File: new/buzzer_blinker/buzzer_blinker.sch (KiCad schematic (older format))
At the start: 9 parts

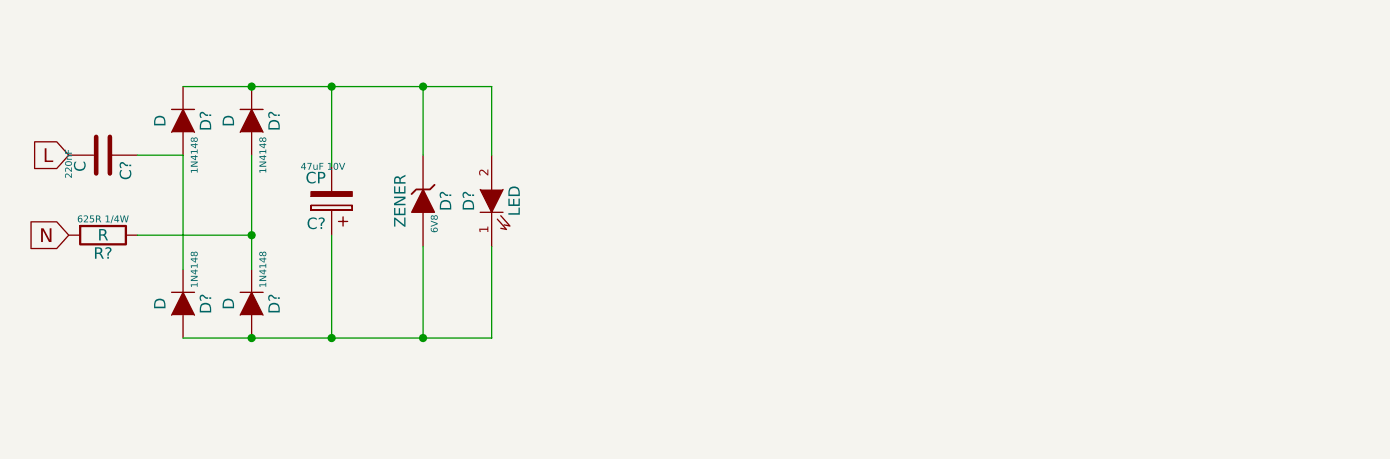
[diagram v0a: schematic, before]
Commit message: .
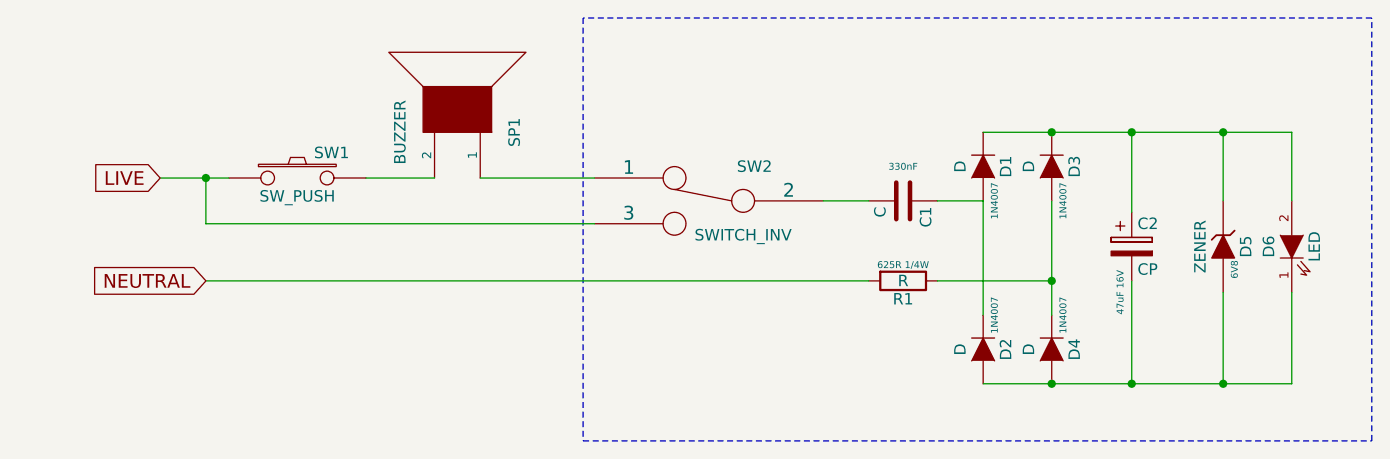
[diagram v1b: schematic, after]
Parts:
- added SP1: BUZZER, symbol SPEAKER
- added SW1: SW_PUSH, symbol SW_PUSH
- added SW2: SWITCH_INV, symbol SWITCH_INV
- C1: renamed from C?; footprint 220nF -> 330nF
- C2: renamed from C?; footprint 47uF 10V -> 47uF 16V
- D1, D2, D3, D4: renamed from D?; footprint 1N4148 -> 1N4007
- gave numbers to parts that had none: 3
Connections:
- net at D1.1 (K), D3.1 (K), D5.1 (K)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: now also C2.1; no longer C2.2
- net at D2.2 (A), D4.2 (A), D5.2 (A)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: now also C2.2; no longer C2.1
- net L: no longer names the net of C1.2
- net L: now also SW2.2
- net N renamed NEUTRAL
- new net: SP1.1, SW2.1
- new net: SP1.2, SW1.2
- new net LIVE: SW1.1, SW2.3
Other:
- moved on the sheet: C1, C2, D1, D2, D3, D4, D5, D6, R1
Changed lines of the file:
@@
 LIBS:contrib
 LIBS:valves
+LIBS:switch_dpdt
+LIBS:buzzer_blinker-cache
 EELAYER 25 0
 EELAYER END
@@
 $EndDescr
 $Comp
-L C C?
+L C C1
 U 1 1 5657A47F
-P 1350 1600
-F 0 "C?" H 1375 1700 50  0000 L CNN
-F 1 "C" H 1375 1500 50  0000 L CNN
-F 2 "220nF" H 1388 1450 30  0000 C CNN
-F 3 "" H 1350 1600 60  0000 C CNN
-	1    1350 1600
-	0    1    1    0
-$EndComp
-$Comp
-L R R?
+P 4850 1800
+F 0 "C1" H 4875 1900 50  0000 L CNN
+F 1 "C" H 4875 1700 50  0000 L CNN
+F 2 "330nF" V 4700 1800 30  0000 C CNN
+F 3 "" H 4850 1800 60  0000 C CNN
+	1    4850 1800
+	0    1    1    0
+$EndComp
+$Comp
+L R R1
 U 1 1 5657A4A7
-P 1350 1950
-F 0 "R?" V 1430 1950 50  0000 C CNN
-F 1 "R" V 1350 1950 50  0000 C CNN
-F 2 "625R 1/4W" V 1280 1950 30  0000 C CNN
-F 3 "" H 1350 1950 30  0000 C CNN
-	1    1350 1950
-	0    1    1    0
-$EndComp
-$Comp
-L D D?
+P 4850 2150
+F 0 "R1" V 4930 2150 50  0000 C CNN
+F 1 "R" V 4850 2150 50  0000 C CNN
+F 2 "625R 1/4W" V 4780 2150 30  0000 C CNN
+F 3 "" H 4850 2150 30  0000 C CNN
+	1    4850 2150
+	0    1    1    0
+$EndComp
+$Comp
+L D D1
 U 1 1 5657A5A6
-P 1700 1450
-F 0 "D?" H 1700 1550 50  0000 C CNN
-F 1 "D" H 1700 1350 50  0000 C CNN
-F 2 "1N4148" H 1850 1500 30  0000 C CNN
-F 3 "" H 1700 1450 60  0000 C CNN
-	1    1700 1450
-	0    1    1    0
-$EndComp
-Wire Wire Line
-	1500 1600 1700 1600
-Wire Wire Line
-	1500 1950 2000 1950
-Wire Wire Line
-	2000 1600 2000 2100
-Connection ~ 2000 1950
-Wire Wire Line
-	1700 1600 1700 2100
-Wire Wire Line
-	1700 1300 3050 1300
-Wire Wire Line
-	1700 2400 3050 2400
-$Comp
-L CP C?
+P 5200 1650
+F 0 "D1" H 5200 1750 50  0000 C CNN
+F 1 "D" H 5200 1550 50  0000 C CNN
+F 2 "1N4007" H 5350 1700 30  0000 C CNN
+F 3 "" H 5200 1650 60  0000 C CNN
+	1    5200 1650
+	0    1    1    0
+$EndComp
+$Comp
+L CP C2
 U 1 1 5657A794
-P 2350 1800
-F 0 "C?" H 2375 1900 50  0000 L CNN
-F 1 "CP" H 2375 1700 50  0000 L CNN
-F 2 "47uF 10V" H 2388 1650 30  0000 C CNN
-F 3 "" H 2350 1800 60  0000 C CNN
-	1    2350 1800
-	-1   0    0    1
-$EndComp
-$Comp
-L ZENER D?
+P 5850 2000
+F 0 "C2" H 5875 2100 50  0000 L CNN
+F 1 "CP" H 5875 1900 50  0000 L CNN
+F 2 "47uF 16V" V 5800 1800 30  0000 C CNN
+F 3 "" H 5850 2000 60  0000 C CNN
+	1    5850 2000
+	1    0    0    -1
+$EndComp
+$Comp
+L ZENER D5
 U 1 1 5657A7EF
-P 2750 1800
-F 0 "D?" H 2750 1900 50  0000 C CNN
-F 1 "ZENER" H 2750 1700 50  0000 C CNN
-F 2 "6V8" H 2850 1850 30  0000 C CNN
-F 3 "" H 2750 1800 60  0000 C CNN
-	1    2750 1800
-	0    1    1    0
-$EndComp
-$Comp
-L LED D?
+P 6250 2000
+F 0 "D5" H 6250 2100 50  0000 C CNN
+F 1 "ZENER" H 6250 1900 50  0000 C CNN
+F 2 "6V8" H 6350 2050 30  0000 C CNN
+F 3 "" H 6250 2000 60  0000 C CNN
+	1    6250 2000
+	0    1    1    0
+$EndComp
+$Comp
+L LED D6
 U 1 1 5657A884
-P 3050 1800
-F 0 "D?" H 3050 1900 50  0000 C CNN
-F 1 "LED" H 3050 1700 50  0000 C CNN
-F 2 "" H 3050 1800 60  0000 C CNN
-F 3 "" H 3050 1800 60  0000 C CNN
-	1    3050 1800
+P 6550 2000
+F 0 "D6" H 6550 2100 50  0000 C CNN
+F 1 "LED" H 6550 1900 50  0000 C CNN
+F 2 "" H 6550 2000 60  0000 C CNN
+F 3 "" H 6550 2000 60  0000 C CNN
+	1    6550 2000
 	0    -1   -1   0
 $EndComp
-Wire Wire Line
-	2350 1300 2350 1650
-Connection ~ 2000 1300
-Wire Wire Line
-	2350 2400 2350 1950
-Connection ~ 2000 2400
-Wire Wire Line
-	2750 1300 2750 1600
-Connection ~ 2350 1300
-Wire Wire Line
-	3050 1300 3050 1600
-Connection ~ 2750 1300
-Wire Wire Line
-	2750 2400 2750 2000
-Connection ~ 2350 2400
-Wire Wire Line
-	3050 2400 3050 2000
-Connection ~ 2750 2400
-Text GLabel 1200 1600 0    60   Input ~ 0
-L
-Text GLabel 1200 1950 0    60   Input ~ 0
-N
-$Comp
-L D D?
+Text GLabel 1800 2150 0    60   Input ~ 0
+NEUTRAL
+$Comp
+L D D2
 U 1 1 5657AEA3
-P 1700 2250
-F 0 "D?" H 1700 2350 50  0000 C CNN
-F 1 "D" H 1700 2150 50  0000 C CNN
-F 2 "1N4148" H 1550 2300 30  0000 C CNN
-F 3 "" H 1700 2250 60  0000 C CNN
-	1    1700 2250
-	0    1    1    0
-$EndComp
-$Comp
-L D D?
+P 5200 2450
+F 0 "D2" H 5200 2550 50  0000 C CNN
+F 1 "D" H 5200 2350 50  0000 C CNN
+F 2 "1N4007" H 5050 2500 30  0000 C CNN
+F 3 "" H 5200 2450 60  0000 C CNN
+	1    5200 2450
+	0    1    1    0
+$EndComp
+$Comp
+L D D3
 U 1 1 5657AEE6
-P 2000 1450
-F 0 "D?" H 2000 1550 50  0000 C CNN
-F 1 "D" H 2000 1350 50  0000 C CNN
-F 2 "1N4148" H 2150 1500 30  0000 C CNN
-F 3 "" H 2000 1450 60  0000 C CNN
-	1    2000 1450
-	0    1    1    0
-$EndComp
-$Comp
-L D D?
+P 5500 1650
+F 0 "D3" H 5500 1750 50  0000 C CNN
+F 1 "D" H 5500 1550 50  0000 C CNN
+F 2 "1N4007" H 5650 1700 30  0000 C CNN
+F 3 "" H 5500 1650 60  0000 C CNN
+	1    5500 1650
+	0    1    1    0
+$EndComp
+$Comp
+L D D4
 U 1 1 5657AF16
-P 2000 2250
-F 0 "D?" H 2000 2350 50  0000 C CNN
-F 1 "D" H 2000 2150 50  0000 C CNN
-F 2 "1N4148" H 1850 2300 30  0000 C CNN
-F 3 "" H 2000 2250 60  0000 C CNN
-	1    2000 2250
-	0    1    1    0
-$EndComp
+P 5500 2450
+F 0 "D4" H 5500 2550 50  0000 C CNN
+F 1 "D" H 5500 2350 50  0000 C CNN
+F 2 "1N4007" H 5350 2500 30  0000 C CNN
+F 3 "" H 5500 2450 60  0000 C CNN
+	1    5500 2450
+	0    1    1    0
+$EndComp
+$Comp
+L SPEAKER SP1
+U 1 1 565D61ED
+P 2900 1400
+F 0 "SP1" H 2800 1650 50  0000 C CNN
+F 1 "BUZZER" H 2800 1150 50  0000 C CNN
+F 2 "" H 2900 1400 60  0000 C CNN
+F 3 "" H 2900 1400 60  0000 C CNN
+	1    2900 1400
+	0    1    -1   0
+$EndComp
+$Comp
+L SW_PUSH SW1
+U 1 1 565D7061
+P 2200 1700
+F 0 "SW1" H 2350 1810 50  0000 C CNN
+F 1 "SW_PUSH" H 2200 1620 50  0000 C CNN
+F 2 "" H 2200 1700 60  0000 C CNN
+F 3 "" H 2200 1700 60  0000 C CNN
+	1    2200 1700
+	1    0    0    -1
+$EndComp
+Text GLabel 1600 1700 0    60   Input ~ 0
+LIVE
+Wire Wire Line
+	5000 1800 5200 1800
+Wire Wire Line
+	5000 2150 5500 2150
+Wire Wire Line
+	5500 1800 5500 2300
+Connection ~ 5500 2150
+Wire Wire Line
+	5200 1800 5200 2300
+Wire Wire Line
+	5200 1500 6550 1500
+Wire Wire Line
+	5200 2600 6550 2600
+Wire Wire Line
+	5850 1500 5850 1850
+Connection ~ 5500 1500
+Wire Wire Line
+	5850 2600 5850 2150
+Connection ~ 5500 2600
+Wire Wire Line
+	6250 1500 6250 1800
+Connection ~ 5850 1500
+Wire Wire Line
+	6550 1500 6550 1800
+Connection ~ 6250 1500
+Wire Wire Line
+	6250 2600 6250 2200
+Connection ~ 5850 2600
+Wire Wire Line
+	6550 2600 6550 2200
+Connection ~ 6250 2600
+Wire Wire Line
+	1600 1700 1900 1700
+Wire Wire Line
+	2500 1700 2800 1700
+Wire Wire Line
+	3000 1700 3500 1700
+Connection ~ 1800 1700
+Wire Wire Line
+	4500 1800 4700 1800
+Wire Wire Line
+	1800 1700 1800 1900
+Wire Wire Line
+	1800 1900 3500 1900
+$Comp
+L SWITCH_INV SW2
+U 1 1 565DA2AE
+P 4000 1800
+F 0 "SW2" H 3800 1950 50  0000 C CNN
+F 1 "SWITCH_INV" H 3850 1650 50  0000 C CNN
+F 2 "" H 4000 1800 60  0000 C CNN
+F 3 "" H 4000 1800 60  0000 C CNN
+	1    4000 1800
+	-1   0    0    -1
+$EndComp
+Wire Wire Line
+	4700 2150 1800 2150
+Wire Notes Line
+	3450 1000 3450 2850
+Wire Notes Line
+	3450 2850 6900 2850
+Wire Notes Line
+	6900 2850 6900 1000
+Wire Notes Line
+	6900 1000 3450 1000
 $EndSCHEMATC
